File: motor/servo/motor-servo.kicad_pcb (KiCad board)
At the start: 2 copper layers, 36.4 x 35 mm, 50 parts, among them J1 DEBUG, J2 servo, J3 Conn_01x06_MountingPin, J6 satellite, U1 SY8205, U10 THVD1400D, U2 LM66100DCK, U5 RP114x, U7 CH32L103F8U6, U8 INA180A2, U9 THVD1400D

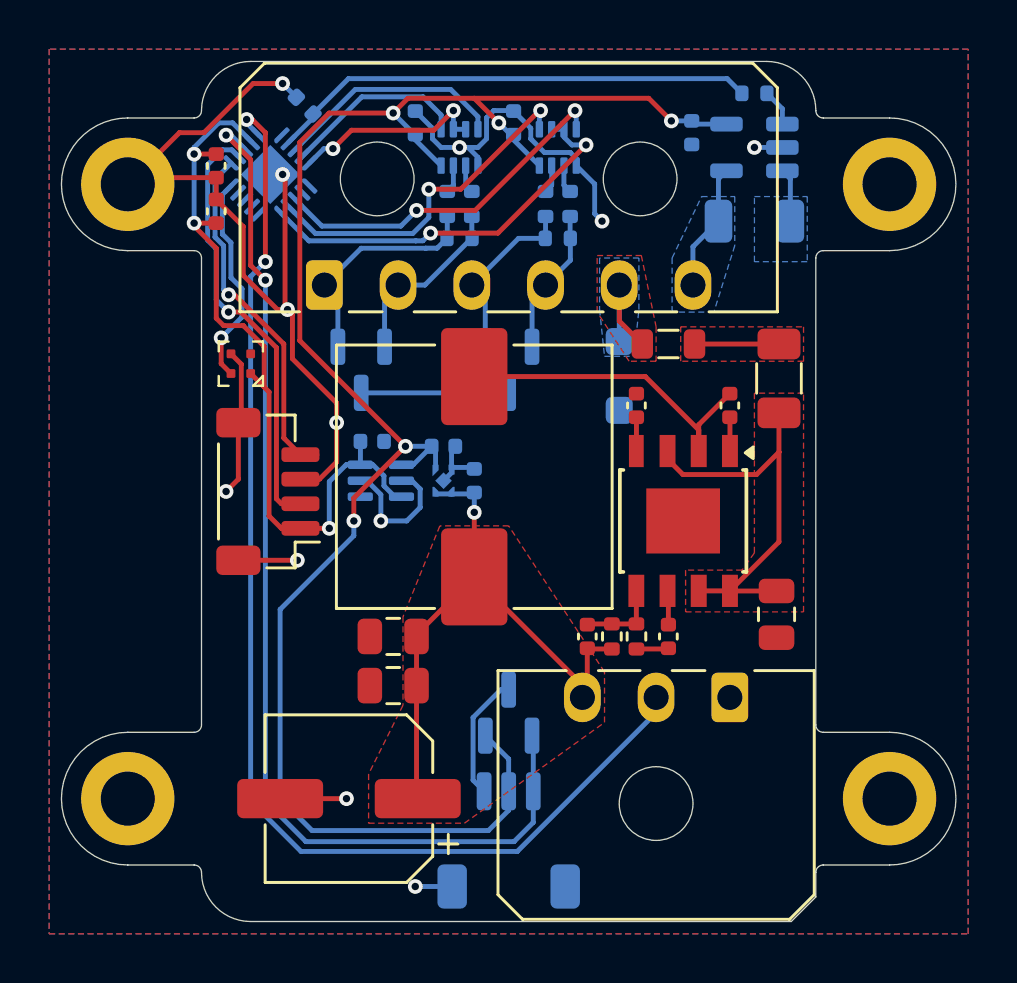
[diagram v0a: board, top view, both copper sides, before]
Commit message: changed buck
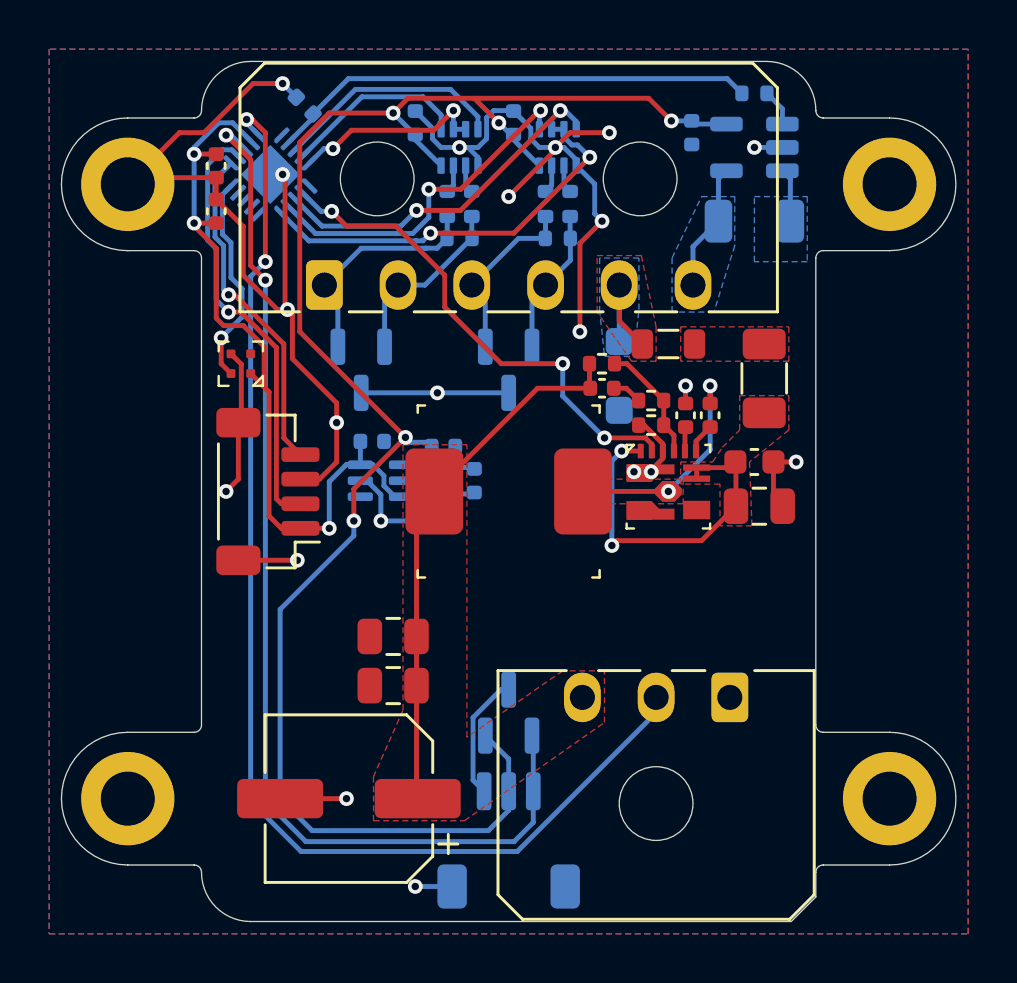
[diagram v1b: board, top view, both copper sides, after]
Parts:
- removed C2: 100n, Capacitor_SMD:C_0402_1005Metric
- removed C3: 1u, Capacitor_SMD:C_0402_1005Metric
- removed C4: C_Small, Capacitor_SMD:C_0402_1005Metric
- removed C5: 100p, Capacitor_SMD:C_0402_1005Metric
- removed C9: 10u, Capacitor_SMD:C_0805_2012Metric
- removed L1: 4.2u, Inductor_SMD:L_Wuerth_HCM-1190
- removed R4: 100k, Resistor_SMD:R_0402_1005Metric
- removed R5: 13k, Resistor_SMD:R_0402_1005Metric
- removed U1: SY8205, Package_SO:Infineon_PG-DSO-8-43
- added C12: 10u (HV), Capacitor_SMD:C_0805_2012Metric, F.Cu at (62.7, 58.1)
- added C15: 1u (HV), Capacitor_SMD:C_0603_1608Metric, F.Cu at (62.5, 56.3)
- added C16: 100n, Capacitor_SMD:C_0402_1005Metric, F.Cu at (60.7, 54.4)
- added C17: 2.2u, Capacitor_SMD:C_0402_1005Metric, F.Cu at (59.7, 54.4)
- added C18: 22p, Capacitor_SMD:C_0402_1005Metric, F.Cu at (56.3, 53.3)
- added L2: 2u, misc:0630CDMCD_DS, F.Cu at (52.5, 57.5)
- added R11: 150k, Resistor_SMD:R_0402_1005Metric, F.Cu at (58.3, 53.8)
- added R13: 100k, Resistor_SMD:R_0402_1005Metric, F.Cu at (56.3, 52.3)
- added R15: 13k, Resistor_SMD:R_0402_1005Metric, F.Cu at (58.3, 54.8)
- added U3: SY8366H, misc:QFN3x3-12, F.Cu at (59.0, 57.3)
- moved F1 0.60 mm to (62.9, 52.9)
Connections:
- U7 pad 7: unconnected-(U7-PA7-Pad7) -> /PG
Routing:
- net /PG: track 0.00 -> 20.3 mm, vias 0 -> 3
- net GND: track 84.7 -> 100.9 mm, vias 12 -> 21
- net Net-(U1-LX): track 13.7 -> 0.00 mm
- net Net-(U3-LX): track 0.00 -> 9.20 mm, vias 0 -> 2
- net Net-(U3-FB): track 0.00 -> 4.85 mm
- net Net-(F1-Pad1): track 3.44 -> 0.00 mm
- net Net-(U1-FB): track 3.36 -> 0.00 mm
- net VBUS: track 16.7 -> 14.4 mm, vias 0 -> 2
- net Net-(U1-VCC): track 1.39 -> 0.00 mm
- net Net-(U1-SS): track 1.38 -> 0.00 mm
- net Net-(U1-BS): track 1.38 -> 0.00 mm
- net Net-(C18-Pad2): track 0.00 -> 1.22 mm
- net Net-(U3-BS): track 0.00 -> 1.21 mm
- net VDD: track 25.2 -> 24.1 mm, vias 1 -> 0
- net Net-(U3-VCC): track 0.00 -> 0.99 mm
- added copper zone on F.Cu, net Net-(U3-LX)
